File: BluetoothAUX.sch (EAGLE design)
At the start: 26 parts, among them IC1 NE5532D, X2 MINI-USB-SCHIELD-32005-201, X3 STEREOJACK

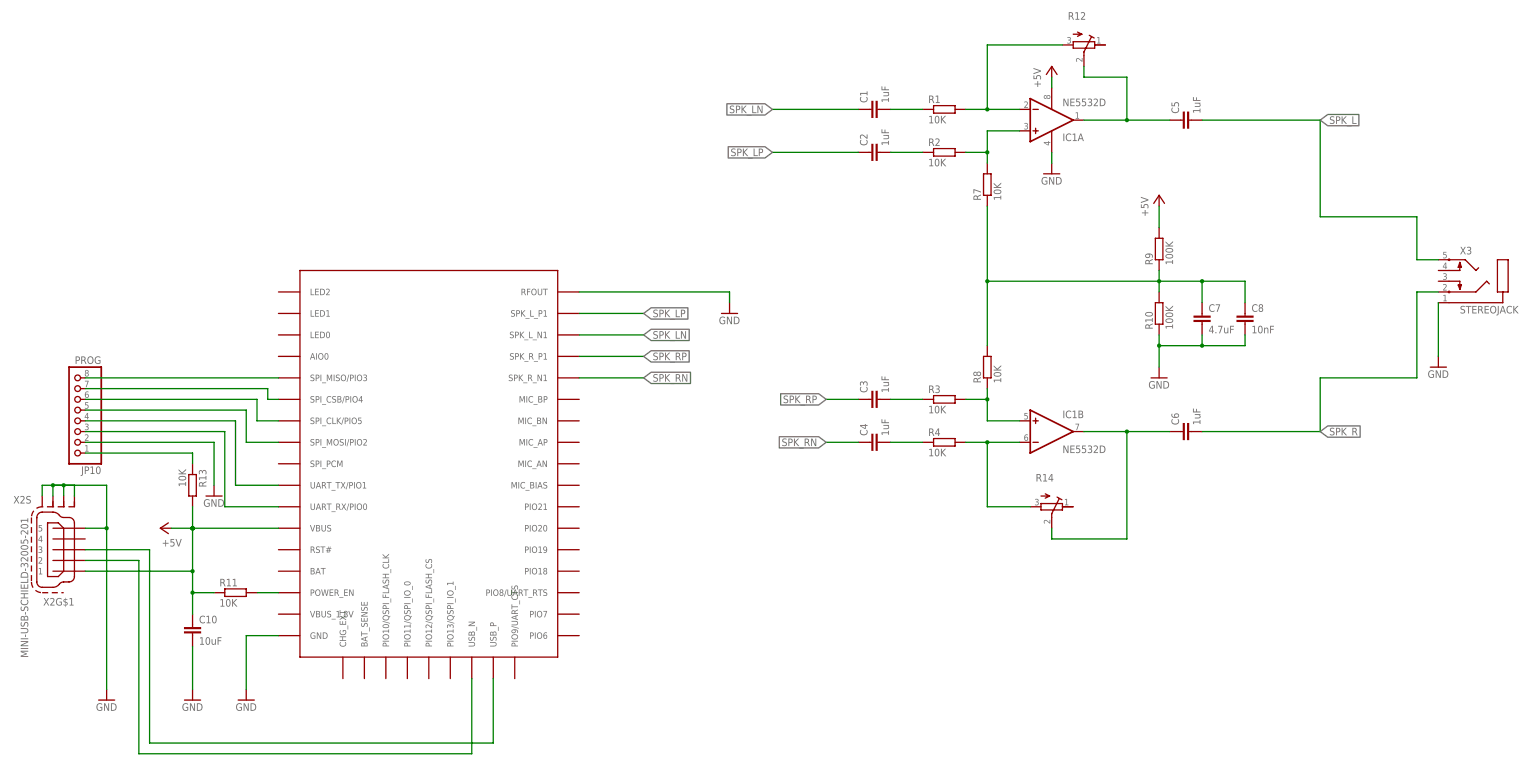
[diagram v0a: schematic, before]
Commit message: TPA6132A
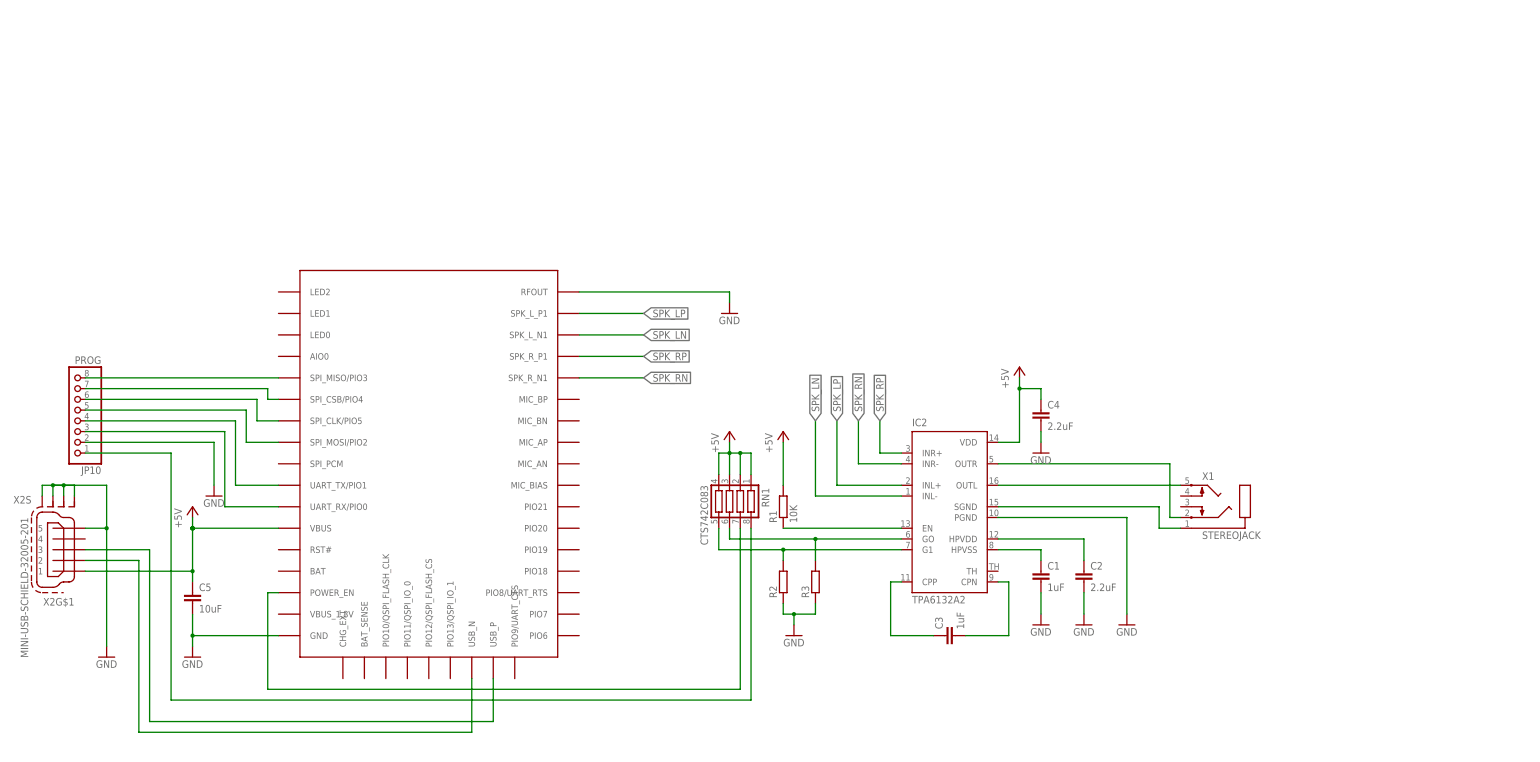
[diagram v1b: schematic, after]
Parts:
- removed C10: 10uF, rcl:C-EUC1206
- removed C6: 1uF, rcl:C-EUC0805
- removed C7: 4.7uF, rcl:C-EUC0805
- removed C8: 10nF, rcl:C-EUC0805
- removed IC1: NE5532D, BT:NE5532D
- removed R10, R9: 100K, rcl:R-EU_R0805
- removed R11, R13, R4, R7, R8: 10K, rcl:R-EU_R0805
- removed R12, R14: (no value), resistor:R-TRIMM3314G
- removed X3: STEREOJACK, adafruit:STEREOJACK
- added IC2: TPA6132A2, texas:TPA6132A2
- added RN1: CTS742C083, resistor-net:CTS742C083
- added X1: STEREOJACK, adafruit:STEREOJACK
- C1, C3: device rcl:C-EUC0805 -> resistor:C-EUC0603
- C2, C4: value 1uF -> 2.2uF; device rcl:C-EUC0805 -> resistor:C-EUC0603
- C5: value 1uF -> 10uF; device rcl:C-EUC0805 -> rcl:C-EUC1206
- R1: device rcl:R-EU_R0805 -> resistor:R-EU_R0603
- R2, R3: value 10K -> (none); device rcl:R-EU_R0805 -> resistor:R-EU_R0603
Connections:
- removed net N$1: IC1A.-IN, R1.2, R12.A
- removed net N$10: C6.1, IC1B.OUT, R14.S
- removed net N$11: C7.1, C8.1, R10.2, R7.1, R8.2, R9.1
- removed net N$2: IC1A.+IN, R2.2, R7.2
- removed net N$3: IC1B.-IN, R14.A, R4.2
- removed net N$4: IC1B.+IN, R3.2, R8.1
- removed net N$5: C1.2, R1.1
- removed net N$6: C2.2, R2.1
- removed net N$7: C3.2, R3.1
- removed net N$8: C4.2, R4.1
- removed net N$9: C5.1, IC1A.OUT, R12.S
- removed net SPK_L: C5.2, X3.5
- removed net SPK_R: C6.2, X3.2
- new net N$14: IC2.OUTR, X1.2
- new net N$20: IC2.OUTL, X1.5
- new net N$26: C3.1, IC2.CPP
- new net N$27: C3.2, IC2.CPN
- new net N$28: C1.1, IC2.HPVSS
- new net N$29: C2.1, IC2.HPVDD
- new net N$30: IC2.EN, R1.1
- new net N$31: IC2.GO, R3.2, RN1.6
- new net N$32: IC2.G1, R2.2, RN1.5
- new net SGND: IC2.SGND, X1.1
- net +5V: now also C4.1, C5.1, IC2.VDD, R1.2, RN1.1, RN1.2, RN1.3, RN1.4; no longer C10.1, IC1P.V+, R11.1, R13.2, R9.2
- net COM: now also RN1.8; no longer R13.1
- net GND: now also C1.2, C2.2, C4.2, C5.2, IC2.PGND, R2.1, R3.1; no longer C10.2, C7.2, C8.2, IC1P.V-, R10.1, X3.1
- net N$13: now also RN1.7; no longer R11.2
- net SPK_LN: now also IC2.INL-; no longer C1.1
- net SPK_LP: now also IC2.INL+; no longer C2.1
- net SPK_RN: now also IC2.INR-; no longer C4.1
- net SPK_RP: now also IC2.INR+; no longer C3.1
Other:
- moved on the sheet: C1, C2, C3, C4, C5, R1, R2, R3
